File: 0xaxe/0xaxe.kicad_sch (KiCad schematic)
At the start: 6 parts, among them J2 Conn_01x04, J3 Barrel_Jack_Switch

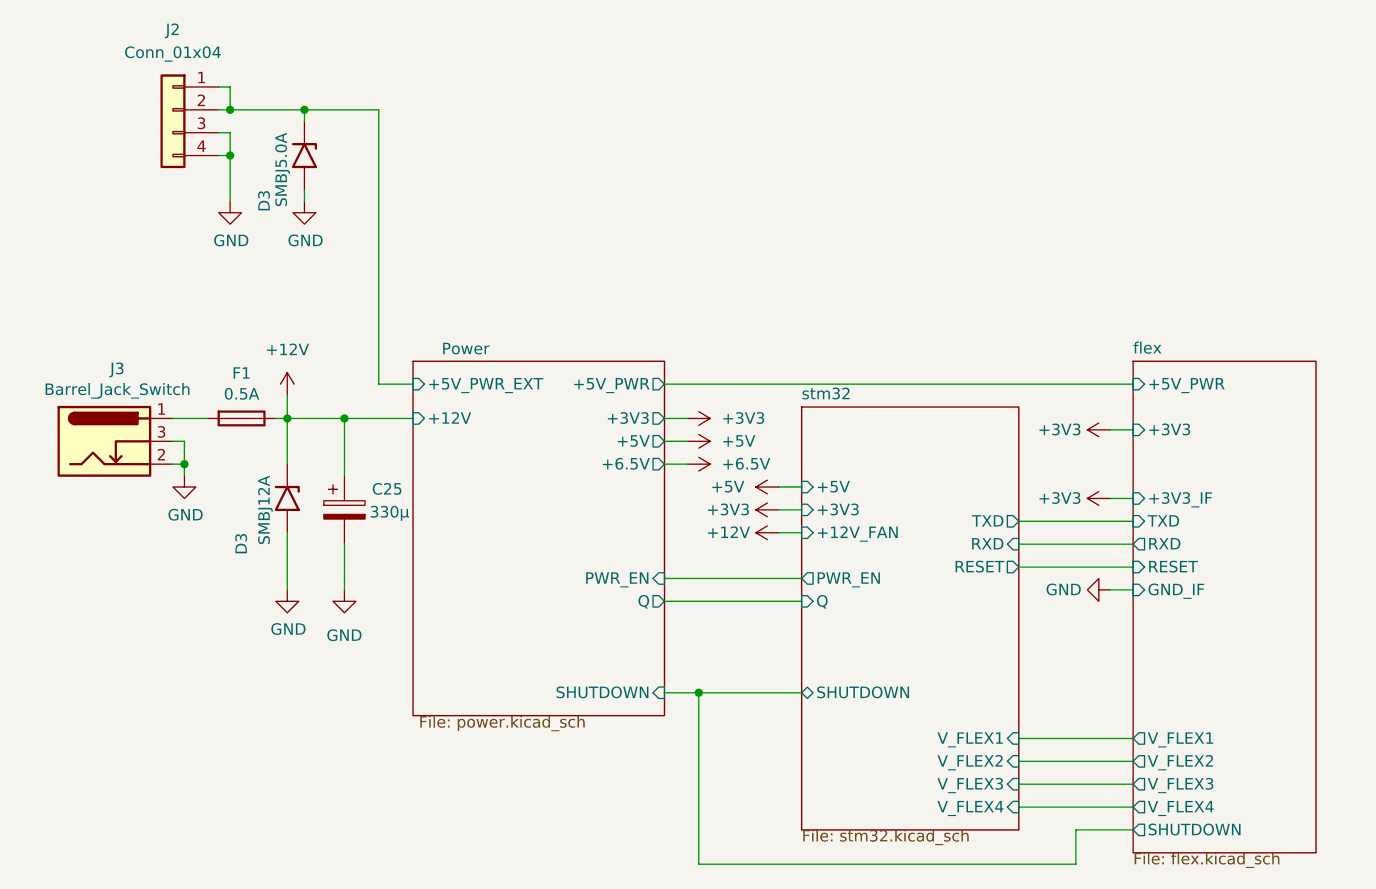
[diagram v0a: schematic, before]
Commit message: fixed couple of things
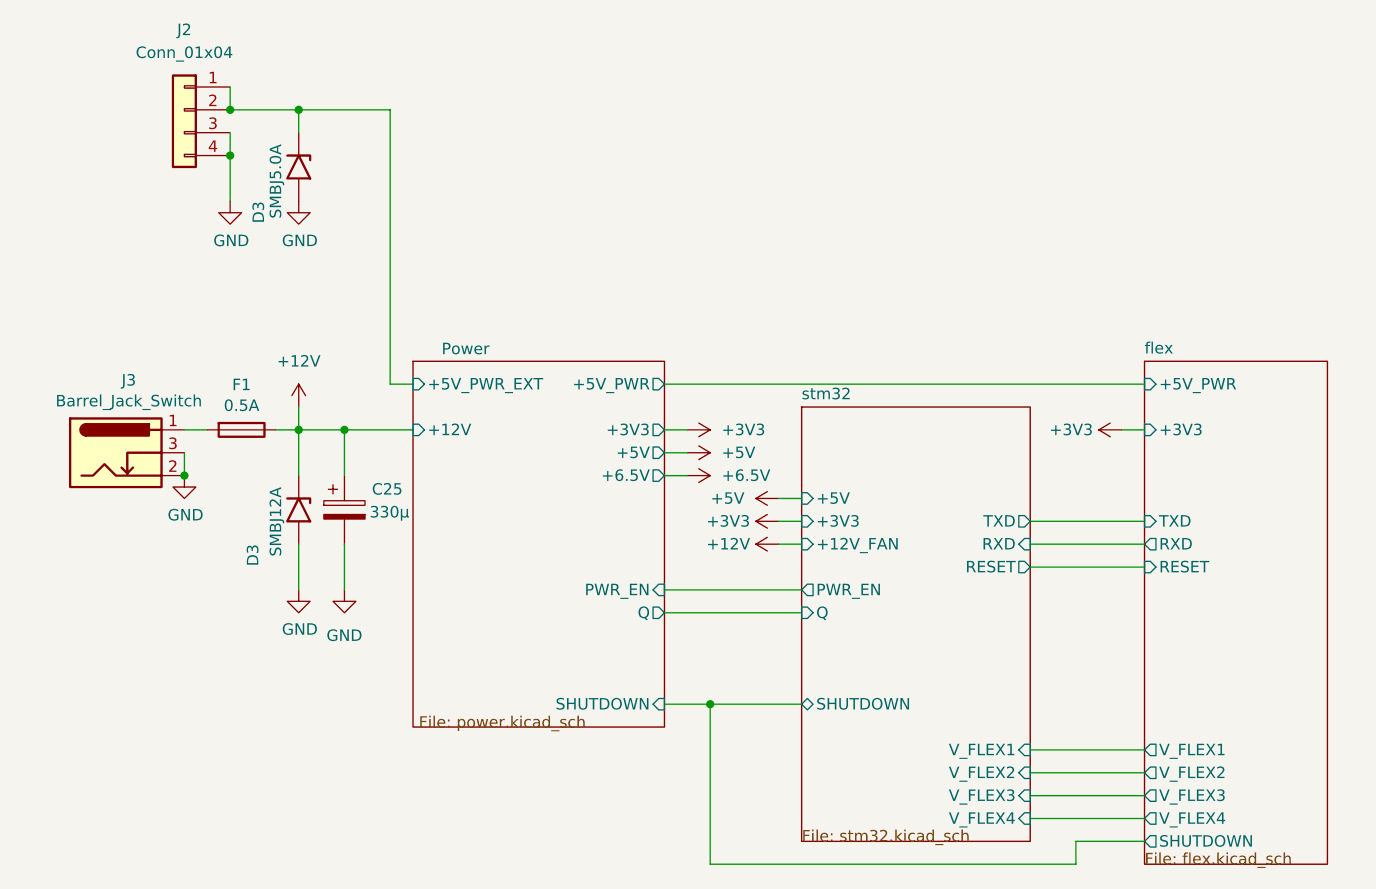
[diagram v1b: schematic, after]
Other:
- sheet flex ports: added none; removed +3V3_IF, GND_IF
- moved on the sheet: D3, F1, J2, J3
